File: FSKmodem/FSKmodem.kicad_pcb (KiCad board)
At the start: 2 copper layers, 27.5 x 14.5 mm, 9 parts, among them IC1 TCM3105, Q1 CSTLS_G

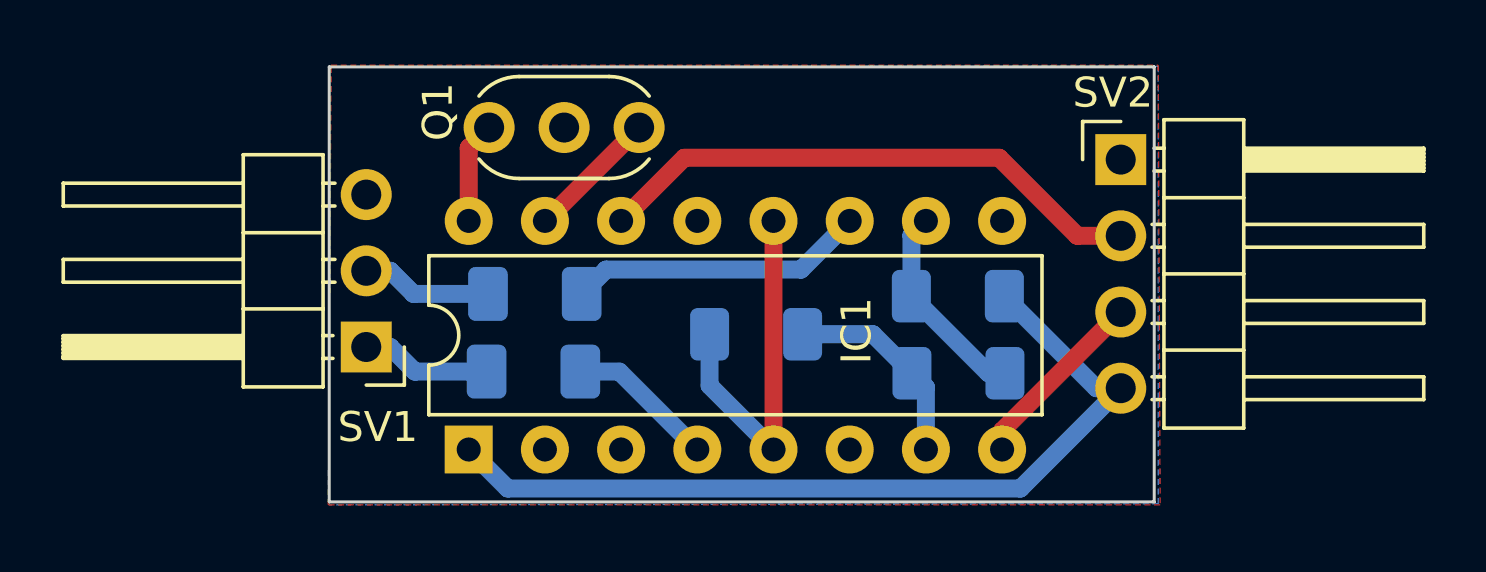
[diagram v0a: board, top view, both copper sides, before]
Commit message: ready for lut
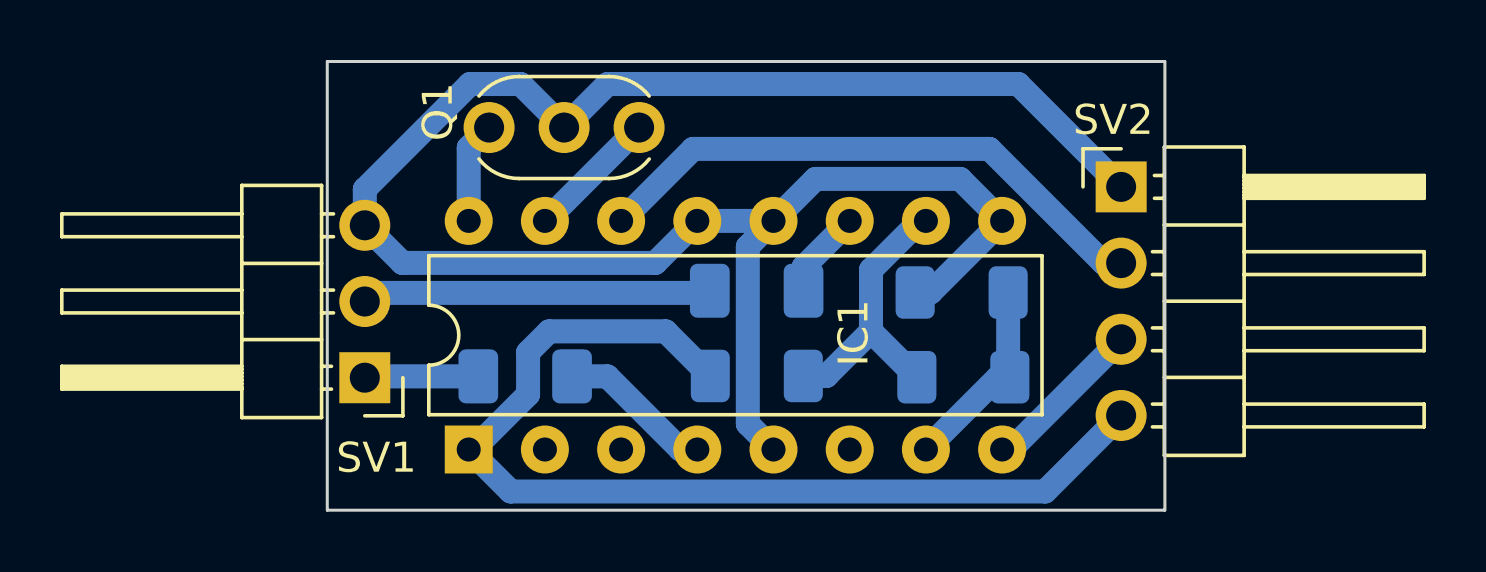
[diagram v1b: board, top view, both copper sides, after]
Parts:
- moved C2 7.40 mm to (116.8, 71.7)
- moved R1 7.21 mm to (116.8, 74.5), turned to 180 degrees
- moved R3 6.99 mm to (123.7, 71.7)
- moved SV1 1.02 mm to (103.8, 74.6)
- moved SV2 0.91 mm to (129.0, 68.2)
- moved C1 0.32 mm to (109.1, 74.5)
- moved R2 0.21 mm to (123.7, 74.5), turned to 180 degrees
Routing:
- net GND: track 12.3 -> 66.2 mm
- net Net-(C2-Pad2): track 4.38 -> 11.6 mm
- net Net-(IC1-TXA): track 9.94 -> 2.97 mm
- net +5V: track 28.8 -> 34.5 mm
- net Net-(IC1-CDL): track 6.89 -> 9.59 mm
- net Net-(IC1-RXD): track 6.22 -> 5.49 mm
- net Net-(IC1-TXD): track 18.6 -> 19.2 mm
- net Net-(C1-Pad2): track 4.35 -> 3.80 mm
- removed copper zone on B.Cu, net GND
- removed copper zone on F.Cu, net GND
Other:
- board size 27.5 x 14.5 mm -> 27.9 x 15 mm
